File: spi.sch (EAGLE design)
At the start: 5 parts, among them IC2 25AA080SN, IC3 25AA080P, X1 2510-

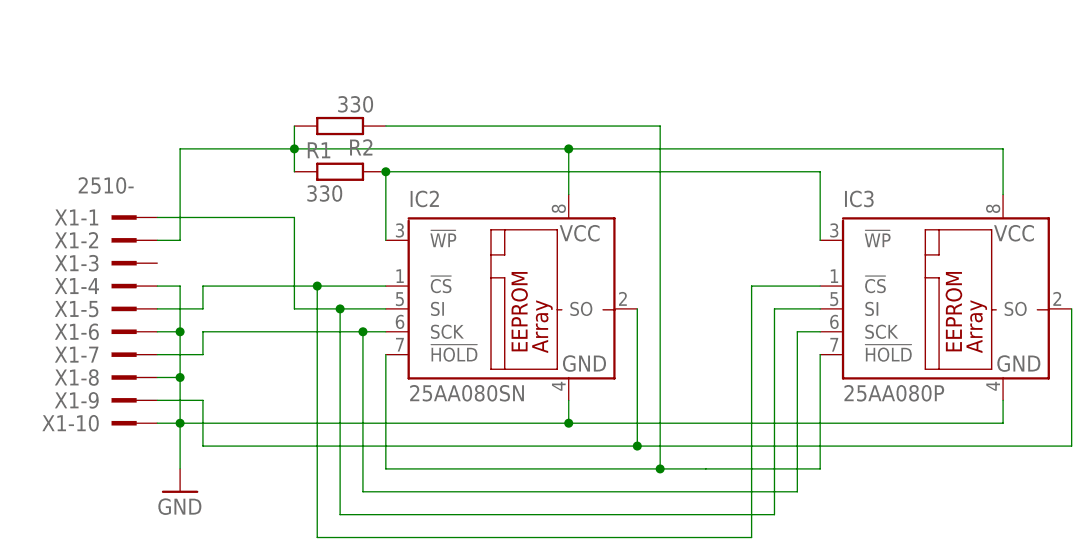
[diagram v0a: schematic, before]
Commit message: Fixed polygon
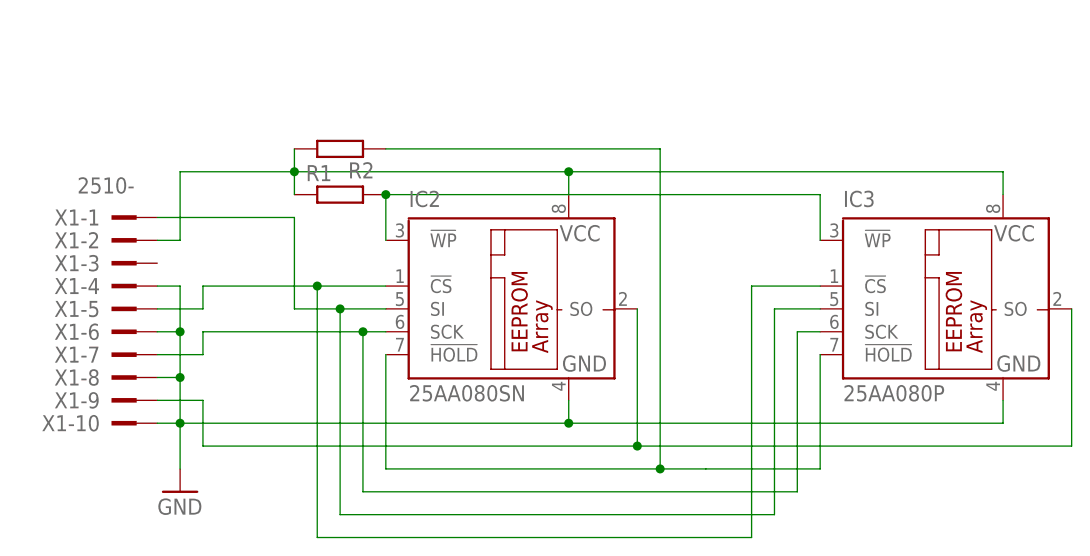
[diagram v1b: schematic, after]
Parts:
- R1, R2: value 330 -> (none); device eagle-ltspice:R0207/10 -> eagle-ltspice:R0204/7
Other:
- moved on the sheet: R1, R2
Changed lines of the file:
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@@
 <layer number="18" name="Vias" color="2" fill="1" visible="no" active="no"/>
 <layer number="19" name="Unrouted" color="6" fill="1" visible="no" active="no"/>
-<layer number="20" name="Dimension" color="15" fill="1" visible="no" active="no"/>
+<layer number="20" name="Dimension" color="24" fill="1" visible="no" active="no"/>
 <layer number="21" name="tPlace" color="7" fill="1" visible="no" active="no"/>
 <layer number="22" name="bPlace" color="7" fill="1" visible="no" active="no"/>
@@
 <layer number="48" name="Document" color="7" fill="1" visible="no" active="no"/>
 <layer number="49" name="Reference" color="7" fill="1" visible="no" active="no"/>
-<layer number="51" name="tDocu" color="6" fill="9" visible="no" active="no"/>
+<layer number="51" name="tDocu" color="7" fill="1" visible="no" active="no"/>
 <layer number="52" name="bDocu" color="7" fill="1" visible="no" active="no"/>
 <layer number="88" name="SimResults" color="9" fill="1" visible="yes" active="yes"/>
@@
 <part name="IC3" library="microchip" library_urn="urn:adsk.eagle:library:294" deviceset="25*" device="P" package3d_urn="urn:adsk.eagle:package:20796/2" technology="AA080"/>
 <part name="X1" library="con-3m" library_urn="urn:adsk.eagle:library:119" deviceset="2510-" device="" package3d_urn="urn:adsk.eagle:package:5571/1"/>
-<part name="R1" library="eagle-ltspice" library_urn="urn:adsk.eagle:library:217" deviceset="R" device="0207/10" package3d_urn="urn:adsk.eagle:package:13275/1" value="330"/>
-<part name="R2" library="eagle-ltspice" library_urn="urn:adsk.eagle:library:217" deviceset="R" device="0207/10" package3d_urn="urn:adsk.eagle:package:13275/1" value="330"/>
+<part name="R1" library="eagle-ltspice" library_urn="urn:adsk.eagle:library:217" deviceset="R" device="0204/7" package3d_urn="urn:adsk.eagle:package:13274/1"/>
+<part name="R2" library="eagle-ltspice" library_urn="urn:adsk.eagle:library:217" deviceset="R" device="0204/7" package3d_urn="urn:adsk.eagle:package:13274/1"/>
 <part name="GND1" library="supply1" library_urn="urn:adsk.eagle:library:371" deviceset="GND" device=""/>
 </parts>
@@
 <instance part="X1" gate="-9" x="-15.24" y="55.88"/>
 <instance part="X1" gate="-10" x="-15.24" y="53.34"/>
-<instance part="R1" gate="G$1" x="10.16" y="81.28"/>
-<instance part="R2" gate="G$1" x="10.16" y="86.36" rot="R180"/>
+<instance part="R1" gate="G$1" x="10.16" y="78.74" smashed="yes">
+<attribute name="NAME" x="6.35" y="80.2386" size="1.778" layer="95"/>
+<attribute name="VALUE" x="6.35" y="75.438" size="1.778" layer="96"/>
+</instance>
+<instance part="R2" gate="G$1" x="10.16" y="83.82" rot="R180"/>
 <instance part="GND1" gate="1" x="-7.62" y="45.72"/>
 </instances>
@@
 <segment>
 <pinref part="IC2" gate="G$1" pin="VCC"/>
-<wire x1="35.56" y1="78.74" x2="35.56" y2="83.82" width="0.1524" layer="91"/>
-<wire x1="35.56" y1="83.82" x2="83.82" y2="83.82" width="0.1524" layer="91"/>
+<wire x1="35.56" y1="78.74" x2="35.56" y2="81.28" width="0.1524" layer="91"/>
+<wire x1="35.56" y1="81.28" x2="83.82" y2="81.28" width="0.1524" layer="91"/>
 <pinref part="IC3" gate="G$1" pin="VCC"/>
-<wire x1="83.82" y1="83.82" x2="83.82" y2="78.74" width="0.1524" layer="91"/>
+<wire x1="83.82" y1="81.28" x2="83.82" y2="78.74" width="0.1524" layer="91"/>
 <pinref part="X1" gate="-2" pin="KL"/>
 <wire x1="-10.16" y1="73.66" x2="-7.62" y2="73.66" width="0.1524" layer="91"/>
-<wire x1="-7.62" y1="73.66" x2="-7.62" y2="83.82" width="0.1524" layer="91"/>
-<wire x1="-7.62" y1="83.82" x2="5.08" y2="83.82" width="0.1524" layer="91"/>
-<junction x="35.56" y="83.82"/>
+<wire x1="-7.62" y1="73.66" x2="-7.62" y2="81.28" width="0.1524" layer="91"/>
+<wire x1="-7.62" y1="81.28" x2="5.08" y2="81.28" width="0.1524" layer="91"/>
+<junction x="35.56" y="81.28"/>
 <pinref part="R1" gate="G$1" pin="1"/>
-<wire x1="5.08" y1="83.82" x2="35.56" y2="83.82" width="0.1524" layer="91"/>
-<wire x1="5.08" y1="81.28" x2="5.08" y2="83.82" width="0.1524" layer="91"/>
-<junction x="5.08" y="83.82"/>
+<wire x1="5.08" y1="81.28" x2="35.56" y2="81.28" width="0.1524" layer="91"/>
+<wire x1="5.08" y1="78.74" x2="5.08" y2="81.28" width="0.1524" layer="91"/>
+<junction x="5.08" y="81.28"/>
 <pinref part="R2" gate="G$1" pin="2"/>
-<wire x1="5.08" y1="86.36" x2="5.08" y2="83.82" width="0.1524" layer="91"/>
+<wire x1="5.08" y1="83.82" x2="5.08" y2="81.28" width="0.1524" layer="91"/>
 </segment>
 </net>
@@
 <wire x1="63.5" y1="60.96" x2="63.5" y2="48.26" width="0.1524" layer="91"/>
 <pinref part="R2" gate="G$1" pin="1"/>
-<wire x1="15.24" y1="86.36" x2="45.72" y2="86.36" width="0.1524" layer="91"/>
-<wire x1="45.72" y1="86.36" x2="45.72" y2="48.26" width="0.1524" layer="91"/>
+<wire x1="15.24" y1="83.82" x2="45.72" y2="83.82" width="0.1524" layer="91"/>
+<wire x1="45.72" y1="83.82" x2="45.72" y2="48.26" width="0.1524" layer="91"/>
 <junction x="45.72" y="48.26"/>
 </segment>
@@
 <pinref part="IC2" gate="G$1" pin="!WP"/>
 <pinref part="R1" gate="G$1" pin="2"/>
-<wire x1="15.24" y1="73.66" x2="15.24" y2="81.28" width="0.1524" layer="91"/>
+<wire x1="15.24" y1="73.66" x2="15.24" y2="78.74" width="0.1524" layer="91"/>
 <pinref part="IC3" gate="G$1" pin="!WP"/>
-<wire x1="63.5" y1="73.66" x2="63.5" y2="81.28" width="0.1524" layer="91"/>
-<wire x1="63.5" y1="81.28" x2="15.24" y2="81.28" width="0.1524" layer="91"/>
-<junction x="15.24" y="81.28"/>
-</segment>
-</net>
+<wire x1="63.5" y1="73.66" x2="63.5" y2="78.74" width="0.1524" layer="91"/>
+<wire x1="63.5" y1="78.74" x2="15.24" y2="78.74" width="0.1524" layer="91"/>
+<junction x="15.24" y="78.74"/>
+</segment>
+</net>

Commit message: Добавлены конденсаторы по питанию
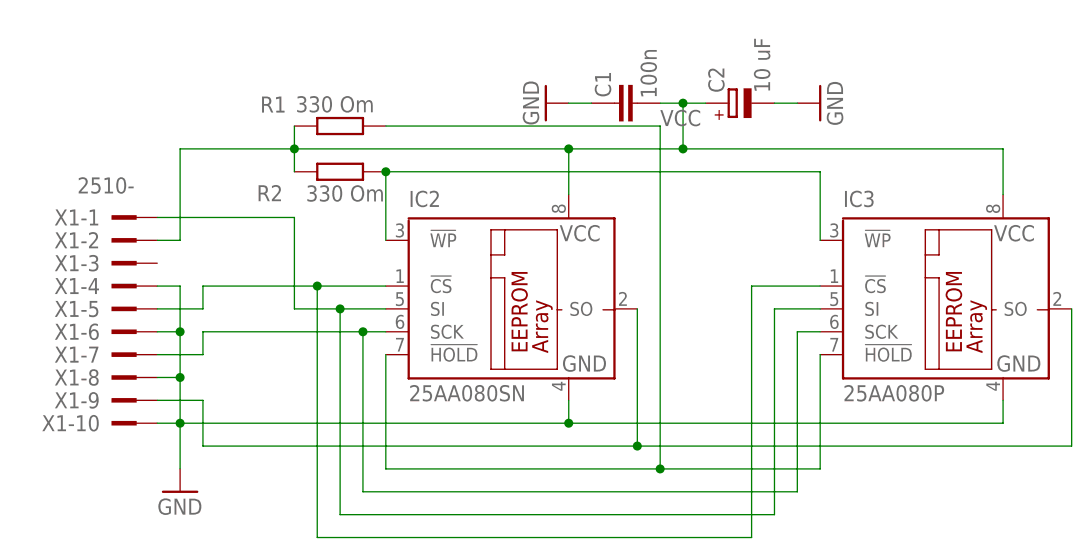
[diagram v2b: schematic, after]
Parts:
- added C1: 100n, resistor:C-EUC0805K
- added C2: 10 uF, resistor:CPOL-EUSMCD
- R1, R2: value (none) -> 330 Om
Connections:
- net GND: now also C1.2, C2.-
- net VCC: now also C1.1, C2.+
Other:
- moved on the sheet: R1, R2
